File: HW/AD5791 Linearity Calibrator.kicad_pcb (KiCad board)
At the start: 4 copper layers, 85 x 68 mm, 63 parts, among them J10 Conn_01x01, J11 ISO OUT, J12 ISO OUT, J2 PWR, J3 REF, J4 REF, J5 REF, J6 REF, J7 Conn_01x01, J8 Conn_01x01, J9 Conn_01x01, SW1 RST, U1 Pico, U11 7533, U12 ADuM1201AR, U2 AD5791BRUZ, U3 LM399, U5 OPA189, U6 OPA189, U7 OPA2140, U8 78L15, U9 79L15

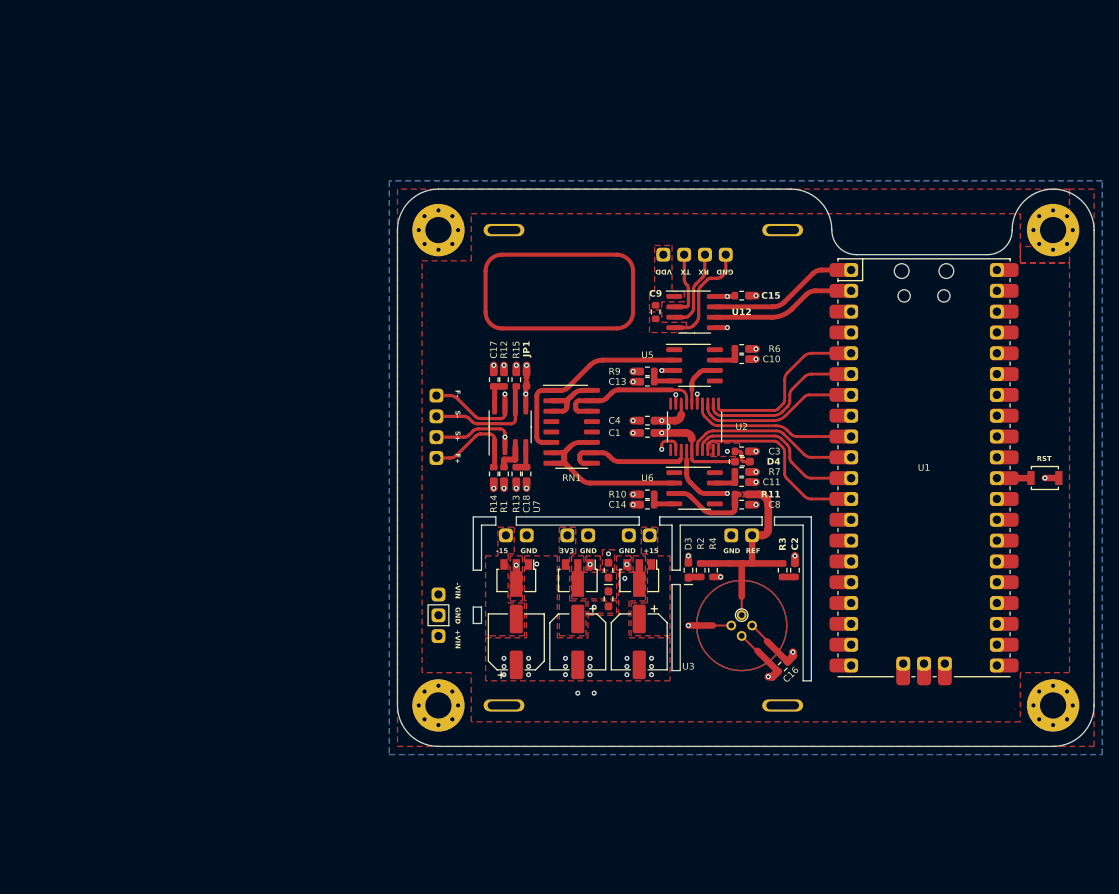
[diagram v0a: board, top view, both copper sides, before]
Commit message: rearranged files
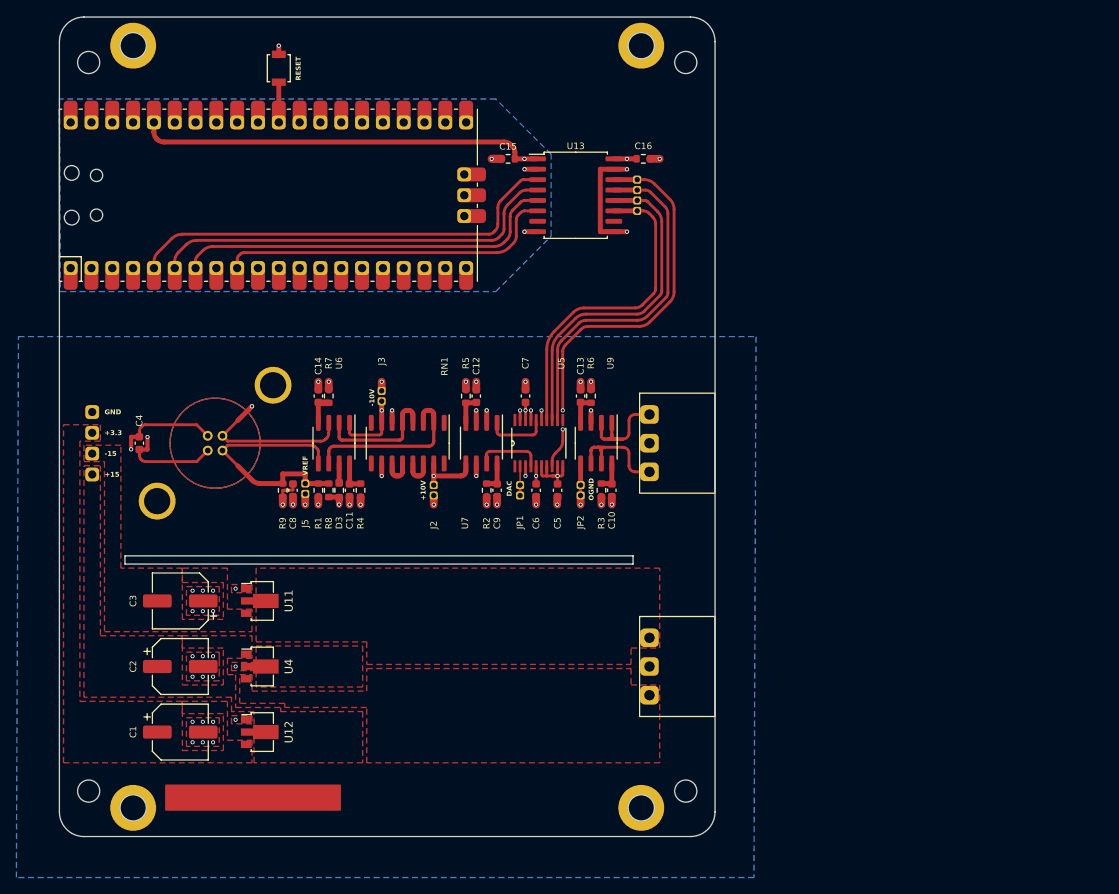
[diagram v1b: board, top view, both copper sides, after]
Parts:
- removed C17, C18: 10uF, Resistor_SMD:R_0603_1608Metric
- removed D1, D2, D4: 5819, Resistor_SMD:R_0603_1608Metric_Pad0.98x0.95mm_HandSolder
- removed H1, H2, H3, H5: MountingHole_Pad, MountingHole:MountingHole_3.2mm_M3_Pad_Via
- removed J10, J9: Conn_01x01, Connector_PinHeader_2.54mm:PinHeader_1x01_P2.54mm_Vertical
- removed J11, J12: ISO OUT, Connector_PinHeader_2.54mm:PinHeader_1x04_P2.54mm_Vertical
- removed R10, R12, R13: 10R, Resistor_SMD:R_0603_1608Metric
- removed R11: 10K, 0603 Jumper:0603 Jumper
- removed R14, R15: 100K, Resistor_SMD:R_0603_1608Metric
- removed U1: Pico, MCU_RaspberryPi_and_Boards:RPi_Pico_SMD_TH
- removed U2: AD5791BRUZ, AD5791BRUZ:SOP65P640X120-20N
- removed U3: LM399, Package_TO_SOT_THT:Analog_TO-46-4_ThermalShield
- added ? (x2): , , F.Cu at (141.0, 146.5)
- added ?: , , F.Cu at (79.0, 146.5)
- added ? (x2): , , F.Cu at (79.0, 53.5)
- added ? (x2): , , F.Cu at (141.0, 53.5)
- added C12: 100nF, Capacitor_SMD:C_0603_1608Metric, F.Cu at (120.9, 96.2)
- added J1: ~, 100mm template footprints:CTB93HD3, F.Cu at (150.0, 129.2)
- added JP2: GND, Connector_PinHeader_1.27mm:PinHeader_1x02_P1.27mm_Vertical, F.Cu at (133.6, 107.1)
- added R5: 10R, Resistor_SMD:R_0603_1608Metric, F.Cu at (119.6, 96.2)
- added R8: 1K, Resistor_SMD:R_0603_1608Metric, F.Cu at (102.9, 107.8)
- added REF**: MountingHole_2.7mm_M2.5_DIN965, MountingHole:MountingHole_2.7mm_M2.5_DIN965, F.Cu at (73.6, 55.5)
- added REF**: MountingHole_2.7mm_M2.5_DIN965, MountingHole:MountingHole_2.7mm_M2.5_DIN965, F.Cu at (146.4, 144.4)
- added REF**: MountingHole_3.2mm_M3_DIN965_Pad, MountingHole:MountingHole_3.2mm_M3_DIN965_Pad, F.Cu at (79.0, 146.5)
- added REF**: MountingHole_2.7mm_M2.5_DIN965, MountingHole:MountingHole_2.7mm_M2.5_DIN965, F.Cu at (73.6, 144.4)
- added REF**: MountingHole_2.7mm_M2.5_DIN965, MountingHole:MountingHole_2.7mm_M2.5_DIN965, F.Cu at (146.4, 55.5)
- added U10: ADR1399, Package_TO_SOT_THT:Analog_TO-46-4_ThermalShield, F.Cu at (89.9, 102.9)
- added U13: ADuM1400xRW, Package_SO:SOIC-16W_7.5x10.3mm_P1.27mm, F.Cu at (133.0, 71.8)
- added U4: L78L15, Package_TO_SOT_SMD:SOT-89-3, F.Cu at (94.8, 129.2)
- C1, C3: value 10uF -> 100uF; footprint Resistor_SMD:R_0603_1608Metric -> Capacitor_SMD:CP_Elec_6.3x5.4
- C10, C11, C13, C14, C9: value 10uF -> 100nF; footprint Resistor_SMD:R_0603_1608Metric -> Capacitor_SMD:C_0603_1608Metric
- C16: value 1uF -> 10uF
- C2: value 1uF -> 100uF; footprint Resistor_SMD:R_0603_1608Metric -> Capacitor_SMD:CP_Elec_6.3x5.4
- C4: value 10uF -> 1uF; footprint Resistor_SMD:R_0603_1608Metric -> Capacitor_SMD:C_0603_1608Metric
- C5, C6, C7: value 100uF -> 10uF; footprint Capacitor_SMD:CP_Elec_6.3x5.4 -> Capacitor_SMD:C_0603_1608Metric
- C8: value 10nF -> 1uF; footprint Resistor_SMD:R_0603_1608Metric -> Capacitor_SMD:C_0603_1608Metric
- J2: value PWR -> VREFP; footprint Connector_PinHeader_2.54mm:PinHeader_1x03_P2.54mm_Vertical -> Connector_PinHeader_1.27mm:PinHeader_1x02_P1.27mm_Vertical
- J3: value REF -> VREFN; footprint Connector_PinHeader_2.54mm:PinHeader_1x02_P2.54mm_Vertical -> Connector_PinHeader_1.27mm:PinHeader_1x02_P1.27mm_Vertical
- J4: value REF -> ~; footprint Connector_PinHeader_2.54mm:PinHeader_1x02_P2.54mm_Vertical -> 100mm template footprints:CTB93HD3
- J5: value REF -> VREFP; footprint Connector_PinHeader_2.54mm:PinHeader_1x02_P2.54mm_Vertical -> Connector_PinHeader_1.27mm:PinHeader_1x02_P1.27mm_Vertical
- J6: value REF -> SIG; footprint Connector_PinHeader_2.54mm:PinHeader_1x02_P2.54mm_Vertical -> Connector_PinHeader_1.27mm:PinHeader_1x04_P1.27mm_Vertical
- J7: value Conn_01x01 -> PWR; footprint Connector_PinHeader_2.54mm:PinHeader_1x01_P2.54mm_Vertical -> Connector_PinHeader_2.54mm:PinHeader_1x04_P2.54mm_Vertical
- J8: value Conn_01x01 -> VREFN; footprint Connector_PinHeader_2.54mm:PinHeader_1x01_P2.54mm_Vertical -> Connector_PinHeader_1.27mm:PinHeader_1x02_P1.27mm_Vertical
- JP1: value GND BRIDGE -> DACOUT; footprint 0603 Jumper:0603 Jumper -> Connector_PinHeader_1.27mm:PinHeader_1x02_P1.27mm_Vertical
- R1: value R -> 100K
- R2: value 6K8 -> 10R
- R3: value 5R1 -> 10R
- R4: value 100K -> 10R
- R9: value 10R -> 5R1
- REF**: moved to B.Cu
- U11: value 7533 -> L79L15
- U12: value ADuM1201AR -> 7533; footprint Package_SO:SOIC-8_3.9x4.9mm_P1.27mm -> Package_TO_SOT_SMD:SOT-89-3
- U5: value OPA189 -> AD5791BRUZ; footprint Package_SO:SOIC-8_3.9x4.9mm_P1.27mm -> AD5791BRUZ:SOP65P640X120-20N
- U6: value OPA189 -> REFSCALE
- U7: value OPA2140 -> REFBUF
- U8: value 78L15 -> Pico; footprint Package_TO_SOT_SMD:SOT-89-3 -> MCU_RaspberryPi_and_Boards:RPi_Pico_SMD_TH
- U9: value 79L15 -> OUTBUF; footprint Package_TO_SOT_SMD:SOT-89-3 -> Package_SO:SOIC-8_3.9x4.9mm_P1.27mm
- moved SW1 106.0 mm to (96.8, 56.2), turned to -90 degrees
- moved C2 75.9 mm to (84.8, 129.2), turned to 0 degrees
- moved REF** 74.3 mm to (109.0, 71.8), turned to 90 degrees
- moved J8 74.0 mm to (89.0, 102.0), turned to 135 degrees
- moved U12 73.5 mm to (94.8, 137.2)
- moved C3 70.9 mm to (84.8, 121.2), turned to 180 degrees
- moved C1 67.7 mm to (84.8, 137.2), turned to 0 degrees
- moved U8 65.2 mm to (95.5, 71.8), turned to 90 degrees
- moved C16 64.2 mm to (141.2, 67.3), turned to 180 degrees
- moved C4 62.1 mm to (79.8, 102.0), turned to -90 degrees
- moved J7 54.9 mm to (74.0, 98.2)
- moved C8 54.8 mm to (98.5, 107.8), turned to -90 degrees
- moved R7 51.2 mm to (102.9, 96.2), turned to -90 degrees
- moved C11 47.9 mm to (105.4, 107.8), turned to 90 degrees
- moved R9 46.8 mm to (97.2, 107.8), turned to -90 degrees
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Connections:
- C1 pad 1: +15V -> +3.3V
- C10 pad 2: Net-(U5A-V+) -> Net-(U9C-V+)
- C11 pad 2: Net-(U6A-V+) -> Net-(U6C-V+)
- C13 pad 2: Net-(U5A-V-) -> Net-(U9C-V-)
- C14 pad 2: Net-(U6A-V-) -> Net-(U6C-V-)
- C15 pad 1: +3.3V -> GNDD
- C15 pad 2: GND -> +3.3VP
- C16 pad 1: +15V -> GND
- C16 pad 2: -15V -> +3.3V
- C2 pad 1: Net-(C2-Pad1) -> +15V
- C2 pad 2: GNDA -> GND
- C3 pad 1: +3.3V -> GND
- C3 pad 2: GND -> -15V
- C4 pad 1: -15V -> +15V
- C4 pad 2: GND -> -15V
- C5 pad 1: +15V -> +3.3V
- C6 pad 1: GND -> +15V
- C6 pad 2: -15V -> GND
- C7 pad 1: +3.3V -> -15V
- C8 pad 1: /7VREF -> Net-(C8-Pad1)
- C8 pad 2: GNDA -> GND
- C9 pad 1: /ISO_VDD -> GND
- C9 pad 2: /ISO_GND -> Net-(U7C-V+)
- D3 pad 1: Net-(D3-K) -> /+10.5V
- D3 pad 2: /VREFPF -> Net-(D3-A)
- J2 pad 1: Net-(J2-Pin_1) -> /+10.5V
- J3 pad 1: +15V -> /-10.5V
- J4 pad 1: /REF -> Net-(J4-Pin_1)
- J5 pad 1: -15V -> /7VREF
- J6 pad 1: +3.3V -> /ISO ~{LDAC}
- J6 pad 2: GND -> /ISO SDIN
- JP1 pad 1: GND -> /BUFIN
- JP1 pad 2: GNDA -> /BUFIN
- R1 pad 1: /DACOUT -> +15V
- R1 pad 2: Net-(U7A-+) -> /7VREF
- R2 pad 1: /REF -> +15V
- R2 pad 2: Net-(D3-K) -> Net-(U7C-V+)
- R3 pad 1: /REF -> +15V
- R3 pad 2: Net-(C2-Pad1) -> Net-(U9C-V+)
- R4 pad 2: /REF -> Net-(U6C-V+)
- R6 pad 1: +15V -> -15V
- R6 pad 2: Net-(U5A-V+) -> Net-(U9C-V-)
- R7 pad 1: +15V -> -15V
- R7 pad 2: Net-(U6A-V+) -> Net-(U6C-V-)
- R9 pad 1: -15V -> /7VREF
- R9 pad 2: Net-(U5A-V-) -> Net-(C8-Pad1)
- RN1 pad 1: Net-(RN1A-R1.1) -> unconnected-(RN1A-R1.1-Pad1)
- RN1 pad 10: /VREFPS -> Net-(RN1F-R6.1)
- RN1 pad 11: Net-(RN1F-R6.2) -> Net-(RN1E-R5.2)
- RN1 pad 12: unconnected-(RN1E-R5.2-Pad12) -> Net-(RN1E-R5.2)
- RN1 pad 13: unconnected-(RN1D-R4.2-Pad13) -> Net-(RN1C-R3.2)
- RN1 pad 14: /VREFNS -> Net-(RN1C-R3.2)
- RN1 pad 15: /VREFNS -> /+10.5V
- RN1 pad 16: Net-(RN1A-R1.2) -> unconnected-(RN1A-R1.2-Pad16)
- RN1 pad 2: Net-(RN1A-R1.2) -> Net-(RN1B-R2.1)
- RN1 pad 3: Net-(RN1A-R1.2) -> Net-(RN1B-R2.1)
- RN1 pad 4: unconnected-(RN1D-R4.1-Pad4) -> Net-(RN1D-R4.1)
- RN1 pad 5: unconnected-(RN1E-R5.1-Pad5) -> Net-(RN1D-R4.1)
- RN1 pad 6: Net-(RN1A-R1.1) -> Net-(RN1F-R6.1)
- RN1 pad 7: Net-(RN1F-R6.2) -> /-10.5V
- RN1 pad 8: Net-(RN1F-R6.2) -> unconnected-(RN1H-R8.1-Pad8)
- RN1 pad 9: /VREFPS -> unconnected-(RN1H-R8.2-Pad9)
- SW1 pad 1: GND -> GNDD
- U11 pad 2: /3V3IN -> Net-(J1-Pin_1)
- U11 pad 3: +3.3V -> -15V
- U12 pad 1: /ISO_VDD -> GND
- U12 pad 2: /ISO_TX -> +15V
- U12 pad 3: /ISO_RX -> +3.3V
- U5 pad 2: Net-(RN1A-R1.1) -> /BUFIN
- U5 pad 3: GNDA -> /VREFPS
- U5 pad 4: Net-(U5A-V-) -> /VREFPF
- U5 pad 5: unconnected-(U5A-NC-Pad5) -> +15V
- U5 pad 6: /VREFNF -> +3.3V
- U5 pad 7: Net-(U5A-V+) -> +3.3V
- U5 pad 8: unconnected-(U5A-VOS-Pad8) -> /ISO ~{LDAC}
- U6 pad 1: unconnected-(U6A-VOS-Pad1) -> /-10.5V
- U6 pad 2: Net-(RN1F-R6.2) -> Net-(RN1D-R4.1)
- U6 pad 3: /7VREF -> GND
- U6 pad 4: Net-(U6A-V-) -> Net-(U6C-V-)
- U6 pad 5: unconnected-(U6A-NC-Pad5) -> /7VREF
- U6 pad 6: /VREFPF -> Net-(RN1B-R2.1)
- U6 pad 7: Net-(U6A-V+) -> Net-(D3-A)
- U6 pad 8: unconnected-(U6A-VOS-Pad8) -> Net-(U6C-V+)
- U7 pad 1: /FORCE+ -> /VREFNF
- U7 pad 2: /SENSE+ -> /VREFNS
- U7 pad 3: Net-(U7A-+) -> /-10.5V
- U7 pad 5: GNDA -> /+10.5V
- U7 pad 6: /SENSE- -> /VREFPS
- U7 pad 7: /FORCE- -> /VREFPF
- U8 pad 1: +15V -> unconnected-(U8-GPIO0-Pad1)
- U8 pad 2: GND -> unconnected-(U8-GPIO1-Pad2)
- U8 pad 3: Net-(J2-Pin_1) -> GNDD
- U9 pad 1: GND -> Net-(J4-Pin_1)
- U9 pad 2: Net-(J2-Pin_3) -> Net-(J4-Pin_1)
- U9 pad 3: -15V -> /BUFIN
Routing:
- net GNDA: track 151.8 -> 0.00 mm, vias 6 -> 0
- net GND: track 12.7 -> 106.9 mm, vias 35 -> 41
- net /ISO ~{LDAC}: track 0.00 -> 53.2 mm, vias 0 -> 2
- net +3.3VP: track 0.00 -> 50.1 mm, vias 0 -> 1
- net /ISO SDIN: track 0.00 -> 45.7 mm
- net /ISO SCLK: track 0.00 -> 43.9 mm
- net /ISO ~{SYNC}: track 0.00 -> 42.3 mm
- net /~{LDAC}: track 23.0 -> 53.5 mm
- net /SDIN: track 20.6 -> 50.4 mm
- net /REF: track 28.2 -> 0.00 mm
- net Net-(RN1F-R6.2): track 28.1 -> 0.00 mm
- net /DACOUT: track 27.3 -> 0.00 mm, vias 2 -> 0
- net /SCLK: track 20.0 -> 47.2 mm
- net Net-(RN1A-R1.1): track 25.6 -> 0.00 mm
- net /+10.5V: track 0.00 -> 23.2 mm, vias 0 -> 2
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- added copper zone on B.Cu, net GNDD
- added copper zone on In1.Cu, net GNDD
- added copper zone on In2.Cu, net GNDD
- added copper zone on F.Cu, net Net-(J1-Pin_1)
- added copper zone on F.Cu, net Net-(J1-Pin_3)
- removed copper zone on In1.Cu, net +3.3V
- removed copper zone on F.Cu, net /3V3IN
- removed copper zone on F.Cu, net /ISO_GND
- removed copper zone on F.Cu, net /ISO_VDD
- removed copper zone on F.Cu, net Net-(D1-A)
- removed copper zone on In1.Cu, net Net-(D1-A)
- removed copper zone on In2.Cu, net Net-(D1-A)
- removed copper zone on F.Cu, net Net-(J2-Pin_1)
- removed copper zone on In2.Cu, net Net-(J2-Pin_1)
- removed copper zone on F.Cu, net Net-(J2-Pin_3)
- removed copper zone on In2.Cu, net Net-(J2-Pin_3)
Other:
- board size 85 x 68 mm -> 80 x 100 mm
- board text added: "+10V"
- board text added: "+3.3"
- board text added: "-10V"
- board text added: "AD5791 LINEARITY CALIBRATOR v2 NNNI 4123"
- board text added: "CLEAN ALL FLUX!"
- board text added: "DAC"
- board text added: "OGND"
- board text added: "RESET"
- board text added: "VREF"
- board text removed: "+VIN"
- board text removed: "-VIN"
- board text removed: "3V3"
- board text removed: "AD5791 LINEARITY CALIBRATOR NNNI 3132"
- board text removed: "F+"
- board text removed: "F-"
- board text removed: "RST"
- board text removed: "RX"
- board text removed: "S+"
- board text removed: "S-"
- board text removed: "TX"
- board text removed: "VDD"
